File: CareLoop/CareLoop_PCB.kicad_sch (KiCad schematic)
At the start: 0 parts

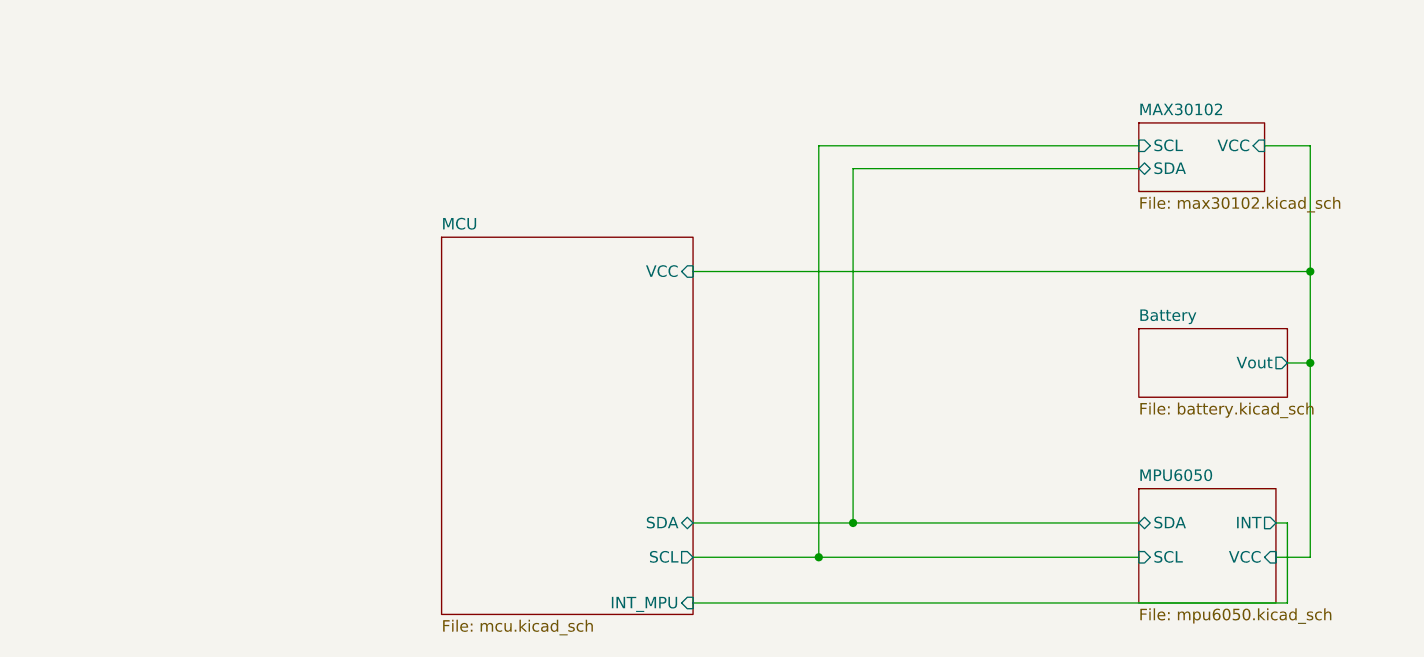
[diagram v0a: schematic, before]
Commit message: updated version
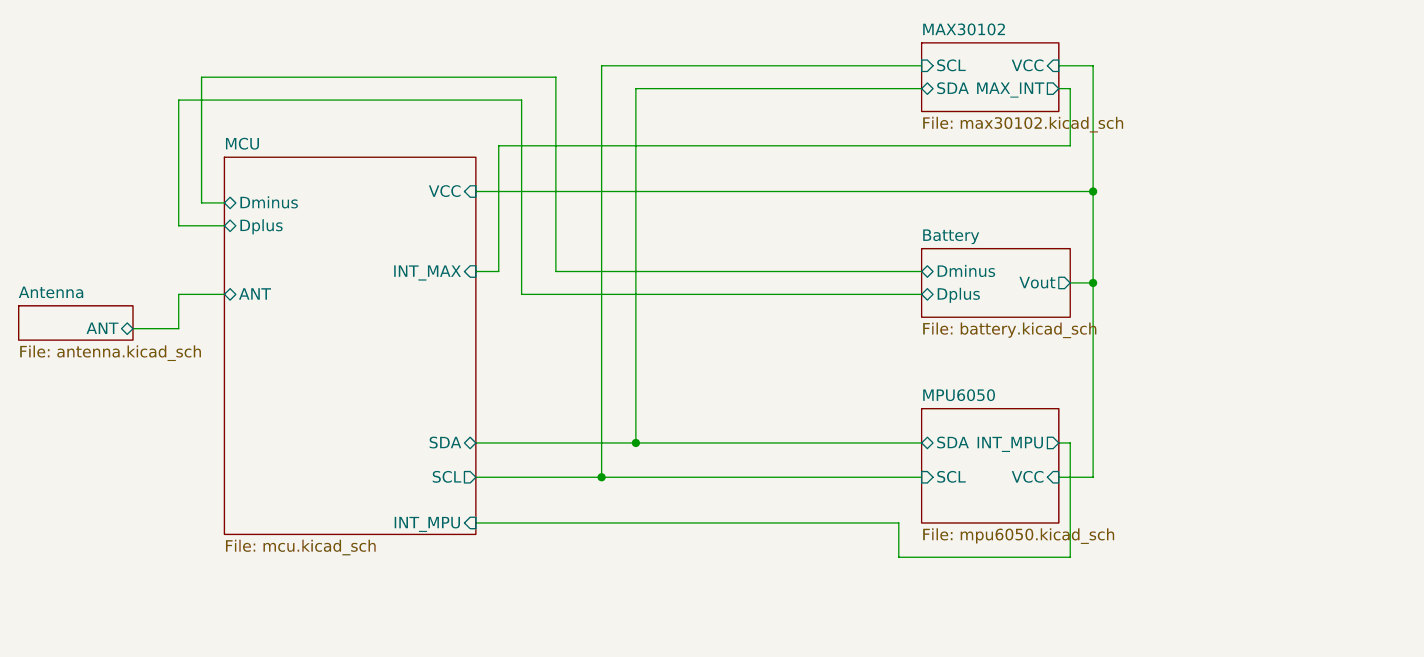
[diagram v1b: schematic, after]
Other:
- added sheet Antenna (antenna.kicad_sch)
- sheet Battery ports: added Dminus, Dplus; removed none
- sheet MAX30102 ports: added MAX_INT; removed none
- sheet MCU ports: added ANT, Dminus, Dplus, INT_MAX; removed none
- sheet MPU6050 ports: added INT_MPU; removed INT
